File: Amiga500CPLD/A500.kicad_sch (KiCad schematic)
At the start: 13 parts, among them J1 Raspberry_Pi_2_3, J2 Conn_01x01, U1 DeniseSocket, U2 DenisePins, U3 XC9572VQ44

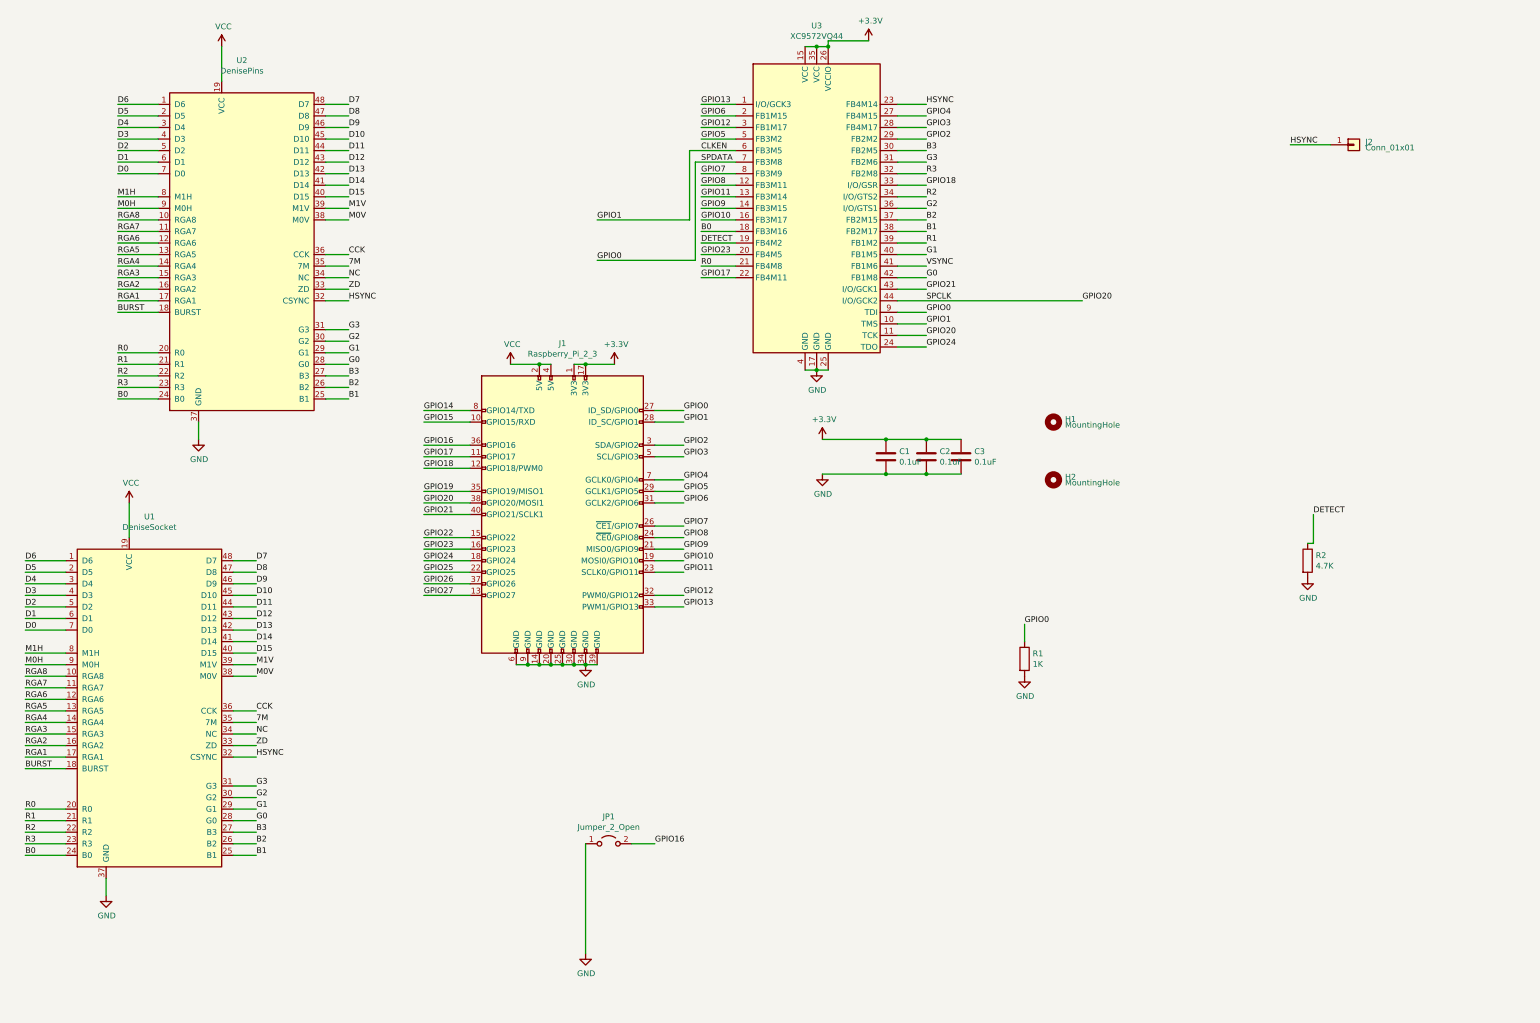
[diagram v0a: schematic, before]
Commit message: Update design to include audio
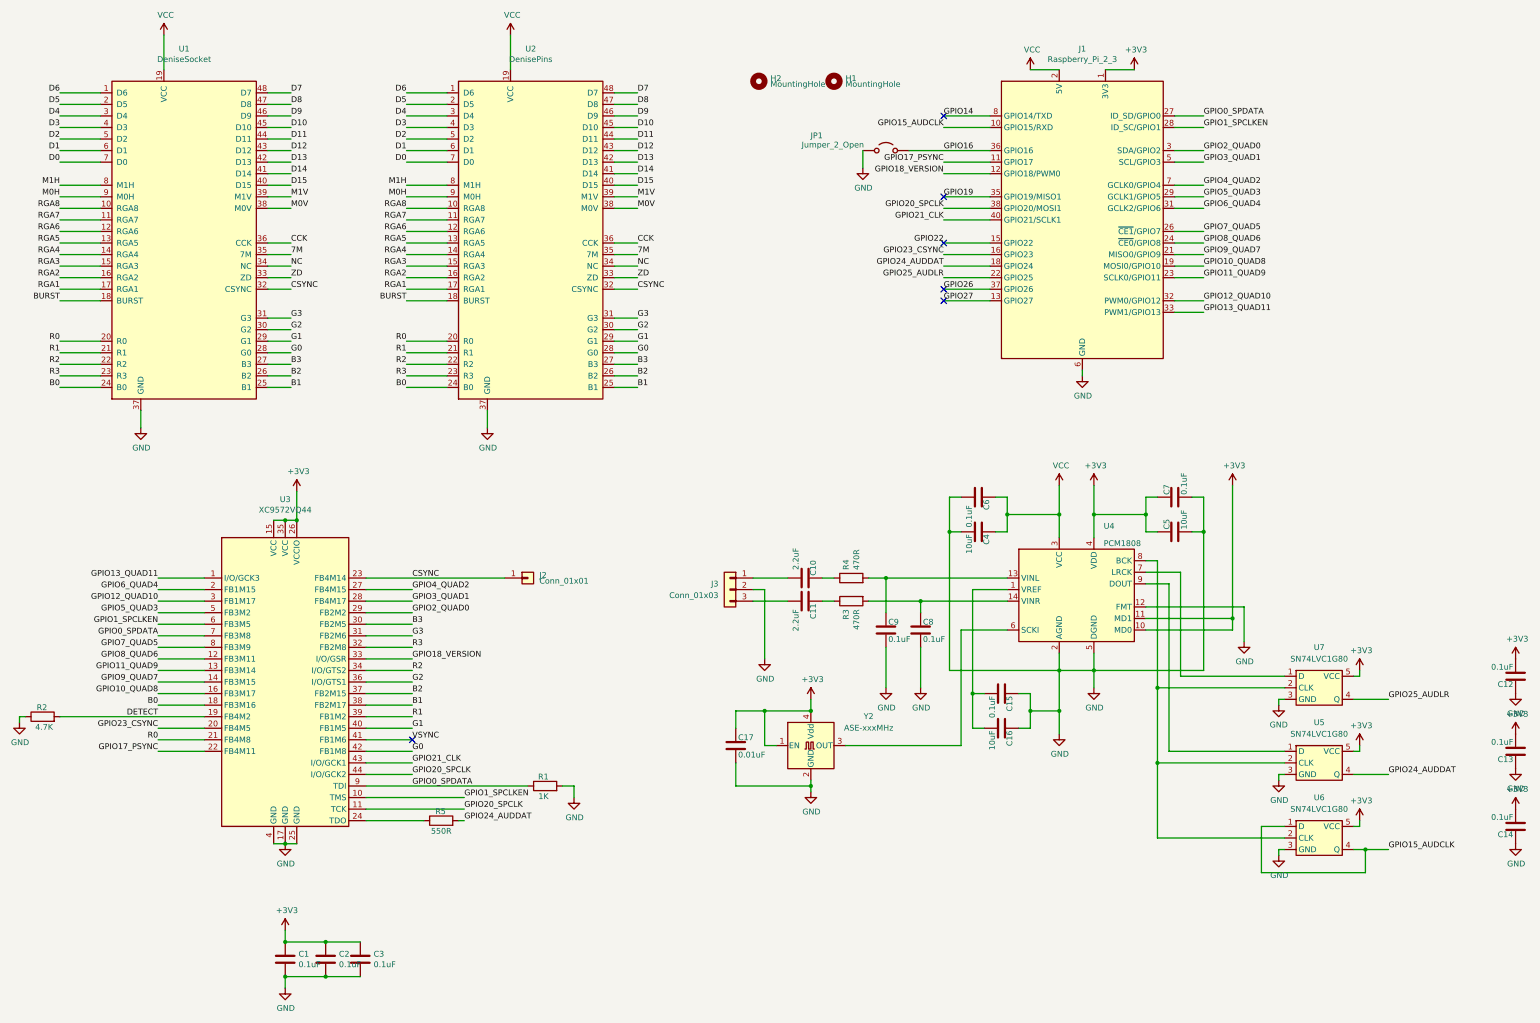
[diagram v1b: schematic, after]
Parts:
- added C10, C11: 2.2uF, Capacitor_SMD:C_0805_2012Metric_Pad1.18x1.45mm_HandSolder, symbol Device:C
- added C12, C13, C14, C15, C6, C7, C8, C9: 0.1uF, Capacitor_SMD:C_0603_1608Metric_Pad1.08x0.95mm_HandSolder, symbol Device:C
- added C16, C4, C5: 10uF, Capacitor_SMD:C_0805_2012Metric_Pad1.18x1.45mm_HandSolder, symbol Device:C
- added C17: 0.01uF, Capacitor_SMD:C_0603_1608Metric_Pad1.08x0.95mm_HandSolder, symbol Device:C
- added J3: Conn_01x03, Connector_PinHeader_2.54mm:PinHeader_1x03_P2.54mm_Horizontal, symbol Connector_Generic:Conn_01x03
- added R3, R4: 470R, Resistor_SMD:R_0603_1608Metric_Pad0.98x0.95mm_HandSolder, symbol Device:R
- added R5: 550R, Resistor_SMD:R_0603_1608Metric_Pad0.98x0.95mm_HandSolder, symbol Device:R
- added U4: PCM1808, Package_SO:TSSOP-14_4.4x5mm_P0.65mm, symbol rgb2hdmi:PCM1808
- added U5, U6, U7: SN74LVC1G80, Package_TO_SOT_SMD:Texas_R-PDSO-G5_DCK-5, symbol rgb2hdmi:SN74LVC1G80
- added Y2: ASE-xxxMHz, Oscillator:Oscillator_SMD_Abracon_ASE-4Pin_3.2x2.5mm, symbol Oscillator:ASE-xxxMHz
- C1, C2, C3: footprint Capacitor_SMD_AKL:C_0603_1608Metric_Pad1.08x0.95mm -> Capacitor_SMD:C_0603_1608Metric_Pad1.08x0.95mm_HandSolder
- J1: footprint Connector_PinSocket_2.54mm:PinSocket_2x20_P2.54mm_Vertical -> Module:Raspberry_Pi_Zero_Socketed_THT_FaceDown_MountingHoles; symbol Connector:Raspberry_Pi_2_3 -> rgb2hdmi:Raspberry_Pi_2_3
- R1, R2: footprint Resistor_SMD_AKL:R_0603_1608Metric_Pad1.05x0.95mm -> Resistor_SMD:R_0603_1608Metric_Pad0.98x0.95mm_HandSolder
- U1: footprint Package_DIP_AKL:DIP-48_W15.24mm_Socket_LongPads -> Package_DIP:DIP-48_W15.24mm_LongPads; symbol rgb2hdmi:AmigaDenise -> rgb2hdmi:AmigaDeniseSocket
- U2: footprint Package_DIP_AKL:DIP-48_W15.24mm_LongPads -> Package_DIP:DIP-48_W15.24mm_LongPads
- U3: footprint Package_QFP_AKL:TQFP-44_10x10mm_P0.8mm -> Package_QFP:TQFP-44_10x10mm_P0.8mm
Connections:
- net +3V3: now also C12.2, C13.2, C14.2, C17.1, C5.1, C7.1, U4.10 (MD0), U4.11 (MD1), U4.4 (VDD), U5.5 (VCC), U6.5 (VCC), U7.5 (VCC), Y2.1 (EN), Y2.4 (Vdd)
- net DETECT: now also R2.2; no longer R2.1
- net GND: now also R2.1, C12.1, C13.1, C14.1, C15.1, C16.1, C17.2, C4.2, C5.2, C6.2, C7.2, C8.2, C9.2, J3.2 (Pin_2), U4.12 (FMT), U4.2 (AGND), U4.5 (DGND), U5.3 (GND), U6.3 (GND), U7.3 (GND), Y2.2 (GND); no longer R2.2
- net VCC: now also C4.1, C6.1, U4.3 (VCC)
- net CLKEN renamed GPIO1_SPCLKEN
- net GPIO0 renamed GPIO0_SPDATA
- net GPIO10 renamed GPIO10_QUAD8
- net GPIO11 renamed GPIO11_QUAD9
- net GPIO12 renamed GPIO12_QUAD10
- net GPIO13 renamed GPIO13_QUAD11
- net GPIO15 renamed GPIO15_AUDCLK
- net GPIO15_AUDCLK: now also U6.1 (D), U6.4 (Q)
- net GPIO17 renamed GPIO17_PSYNC
- net GPIO18 renamed GPIO18_VERSION
- net GPIO2 renamed GPIO2_QUAD0
- net GPIO20 renamed GPIO20_SPCLK
- net GPIO21 renamed GPIO21_CLK
- net GPIO23 renamed GPIO23_CSYNC
- net GPIO24: no longer names the net of U3.24 (TDO)
- net GPIO24: now also R5.1; no longer J1.18 (GPIO24)
- net GPIO25 renamed GPIO25_AUDLR
- net GPIO25_AUDLR: now also U7.4 (Q)
- net GPIO3 renamed GPIO3_QUAD1
- net GPIO4 renamed GPIO4_QUAD2
- net GPIO5 renamed GPIO5_QUAD3
- net GPIO6 renamed GPIO6_QUAD4
- net GPIO7 renamed GPIO7_QUAD5
- net GPIO8 renamed GPIO8_QUAD6
- net GPIO9 renamed GPIO9_QUAD7
- net HSYNC renamed CSYNC
- new net: C11.1, R3.1
- new net: C8.1, R3.2, U4.14 (VINR)
- new net: C15.2, C16.2, U4.1 (VREF)
- new net: C10.2, J3.1 (Pin_1)
- new net: C11.2, J3.3 (Pin_3)
- new net: U4.7 (LRCK), U7.1 (D)
- new net: U4.8 (BCK), U5.2 (CLK), U6.2 (CLK), U7.2 (CLK)
- new net: C10.1, R4.1
- new net: C9.1, R4.2, U4.13 (VINL)
- new net: U4.6 (SCKI), Y2.3 (OUT)
- new net: U4.9 (DOUT), U5.1 (D)
- new net GPIO24_AUDDAT: J1.18 (GPIO24), R5.2, U5.4 (Q)
- no-connect marks 0 -> 6
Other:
- moved on the sheet: C1, C2, C3, H1, H2, J2, R1, R2, U1, U2, U3
